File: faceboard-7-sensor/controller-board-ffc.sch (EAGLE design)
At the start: 8 parts, among them J1 DCJ0202

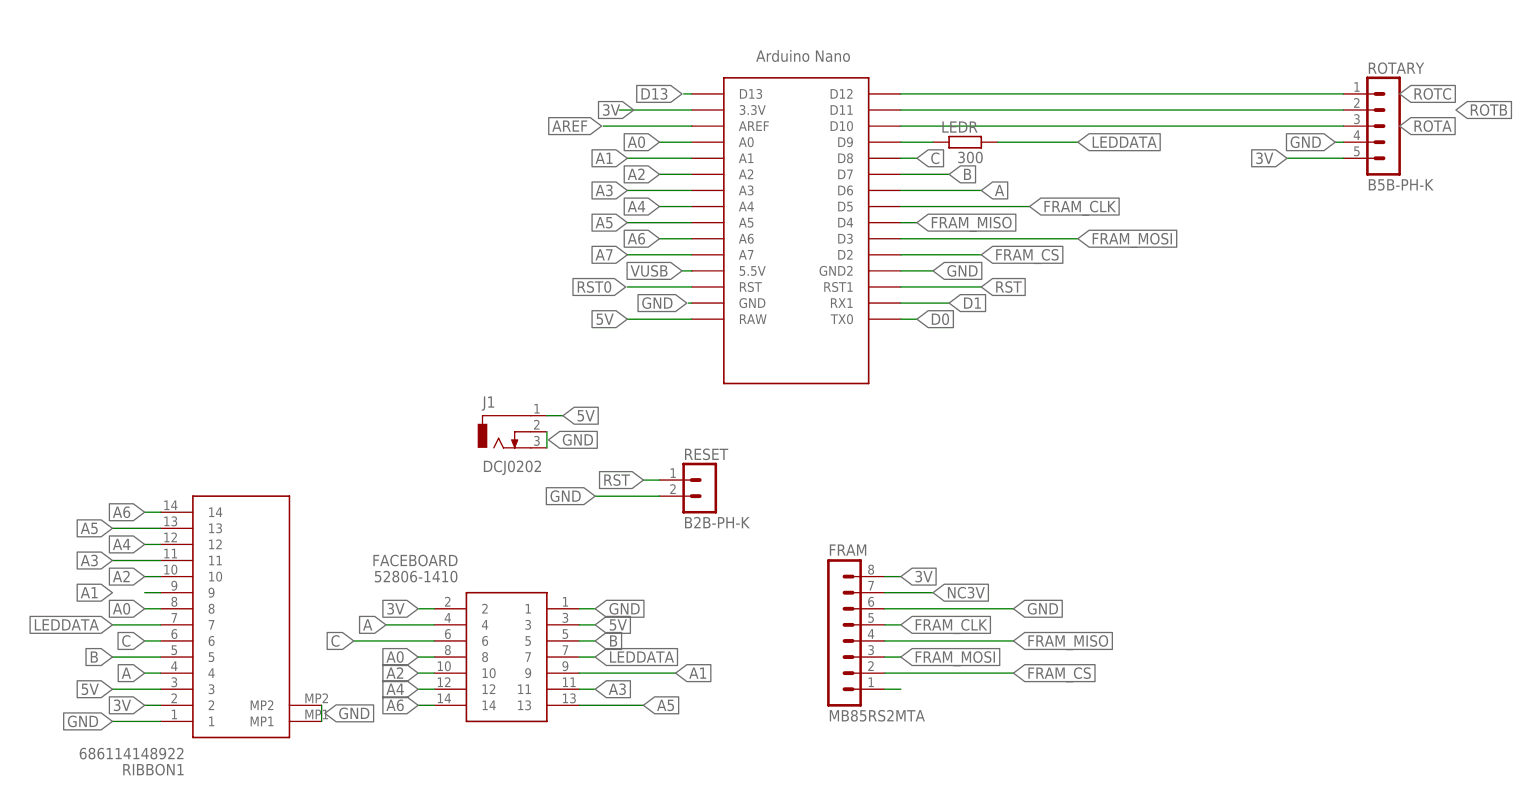
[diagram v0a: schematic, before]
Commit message: redraw schematics
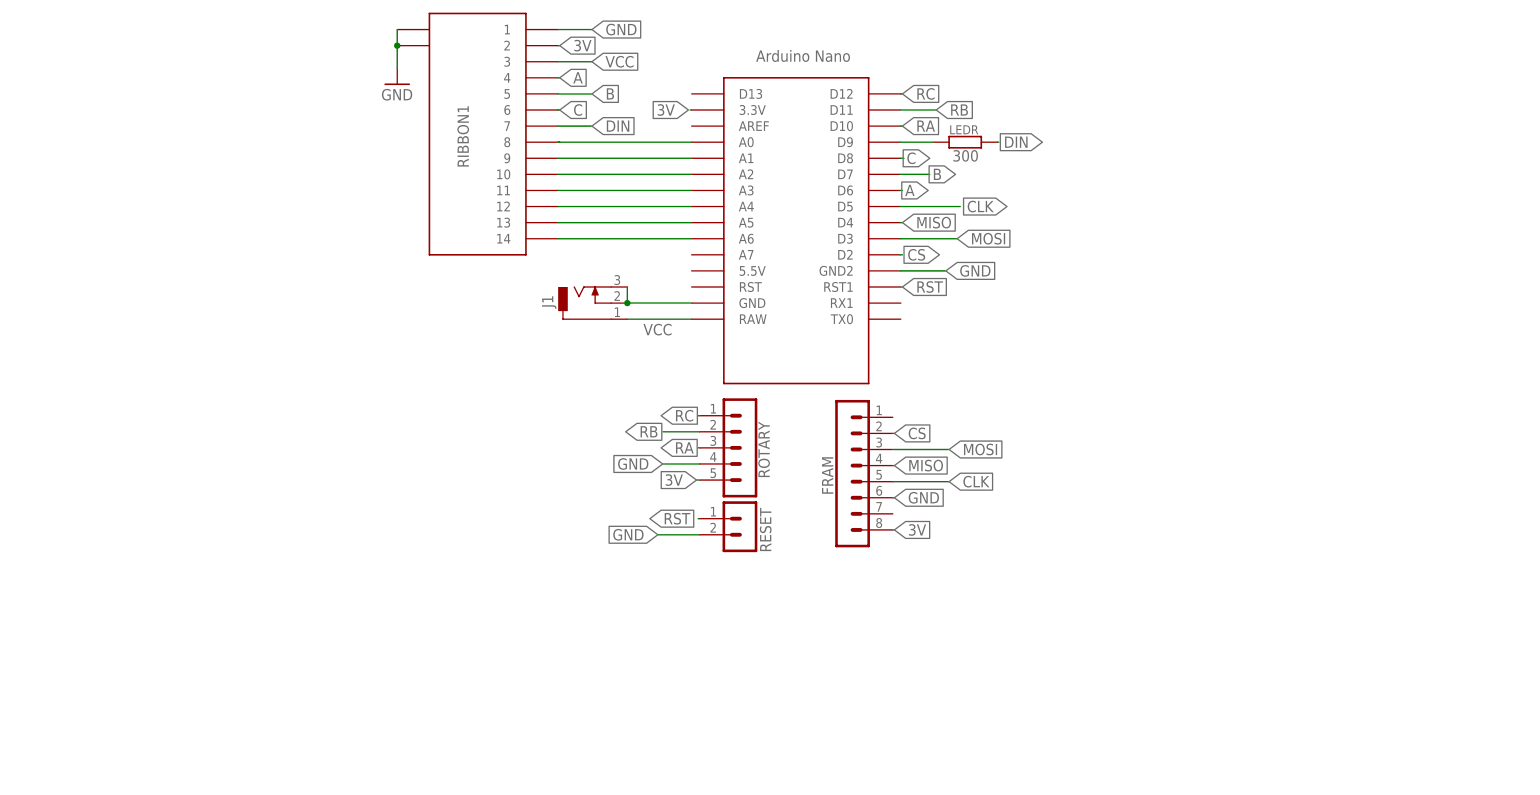
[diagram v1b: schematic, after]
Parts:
- removed FACEBOARD: 52806-1410, 52806-1410:52806-1410
- RIBBON1: value 686114148922 -> (none)
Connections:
- net FRAM_CLK renamed CLK
- net FRAM_CS renamed CS
- net FRAM_MISO renamed MISO
- net FRAM_MOSI renamed MOSI
- net ROTA renamed RA
- net ROTB renamed RB
- net ROTC renamed RC
- removed net 5V: FACEBOARD.3, J1.1, RIBBON1.3, U$1.RAW
- removed net A4: FACEBOARD.12, RIBBON1.12, U$1.A4
- removed net A6: FACEBOARD.14, RIBBON1.14, U$1.A6
- removed net A7: U$1.A7
- removed net AREF: U$1.AREF
- removed net D0: U$1.TX0
- removed net D1: U$1.RX1
- removed net D13: U$1.D13
- removed net LEDDATA: FACEBOARD.7, LEDR.2, RIBBON1.7
- removed net N$8: FRAM.1
- removed net NC3V: FRAM.7
- removed net RST0: U$1.RST
- removed net VUSB: U$1.5.5V
- new net DIN: LEDR.2, RIBBON1.7
- new net N$1: RIBBON1.12, U$1.A4
- new net N$2: RIBBON1.14, U$1.A6
- new net VCC: J1.1, RIBBON1.3, U$1.RAW
- net 3V: no longer FACEBOARD.2
- net A: no longer FACEBOARD.4
- net A0: no longer FACEBOARD.8
- net A1: no longer FACEBOARD.9
- net A2: no longer FACEBOARD.10
- net A3: no longer FACEBOARD.11
- net A5: no longer FACEBOARD.13
- net B: no longer FACEBOARD.5
- net C: no longer FACEBOARD.6
- net GND: no longer FACEBOARD.1
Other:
- moved on the sheet: FRAM, J1, RESET, ROTARY
